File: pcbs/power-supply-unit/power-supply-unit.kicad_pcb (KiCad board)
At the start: 2 copper layers, 34.3 x 83.2 mm, 23 parts, among them J1 BMS_OUTPUT, J2 PWR_CONN_RASPI, J3 PWR_CONN_CTRL, U1 LM2576S-ADJ, U2 LM2576S-ADJ, U3 AMS1117-3.3

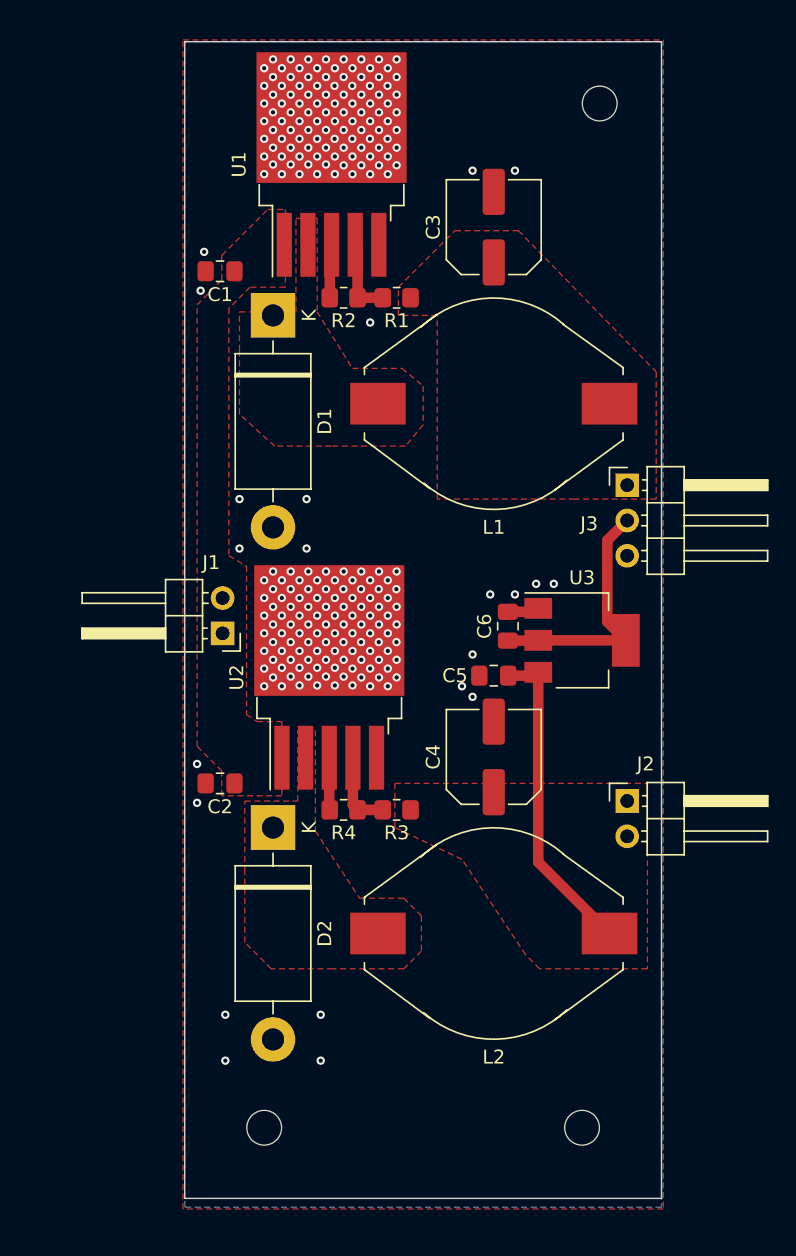
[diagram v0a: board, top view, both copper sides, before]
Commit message: Redesign PWR supply to match real part footprints
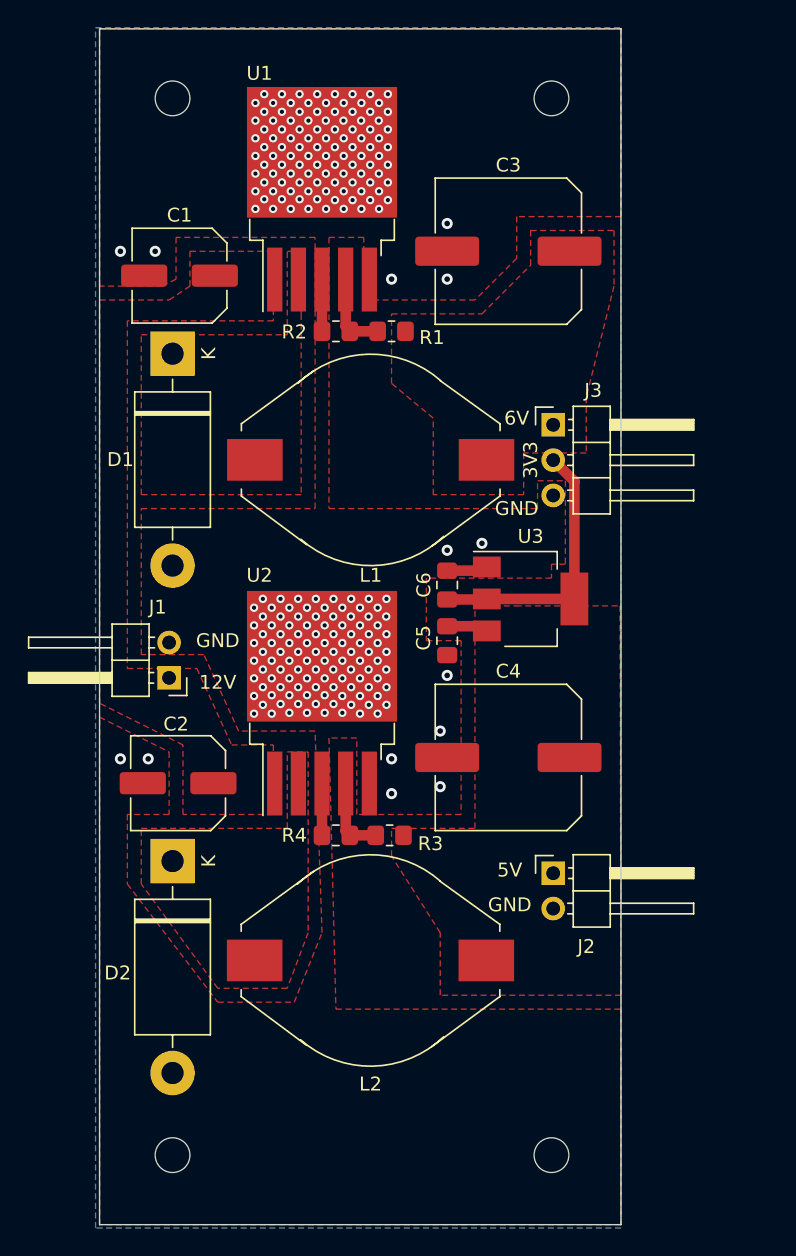
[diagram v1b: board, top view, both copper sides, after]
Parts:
- added REF03: MountingHole_2.5mm, MountingHole:MountingHole_2.5mm, F.Cu at (110.2, 39.0)
- C1, C2: footprint Capacitor_SMD:C_0805_2012Metric_Pad1.18x1.45mm_HandSolder -> Capacitor_SMD:C_Elec_6.3x7.7
- C3, C4: footprint Capacitor_SMD:C_Elec_6.3x7.7 -> Capacitor_SMD:C_Elec_10x10.2
- moved L1 9.73 mm to (124.5, 65.0)
- moved L2 9.07 mm to (124.5, 101.0)
- moved D1 7.73 mm to (110.2, 57.4)
- moved D2 7.62 mm to (110.2, 93.9)
- moved J2 7.44 mm to (137.6, 94.7)
- moved REF02 6.88 mm to (110.2, 115.0)
- moved J3 6.87 mm to (137.6, 62.5)
- moved C6 5.28 mm to (130.0, 74.0)
- moved J1 5.01 mm to (110.0, 80.7)
- moved U3 4.75 mm to (136.0, 75.0)
- moved C5 4.19 mm to (130.0, 78.0), turned to -90 degrees
- moved REF03 3.49 mm to (137.5, 39.0)
- moved C2 3.02 mm to (110.6, 88.2)
- moved REF01 2.95 mm to (137.5, 115.0)
- moved C1 2.93 mm to (110.8, 51.8)
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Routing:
- net +5V: track 23.2 -> 2.99 mm
- net +3V3: track 18.3 -> 19.8 mm
- net GND: track 9.91 -> 10.4 mm, vias 246 -> 238
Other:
- board size 34.3 x 83.2 mm -> 37.5 x 86 mm
- board text added: "12V"
- board text added: "3V3"
- board text added: "5V"
- board text added: "6V"
- board text added: "GND"

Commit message: Fix small errors, add more stitching vias
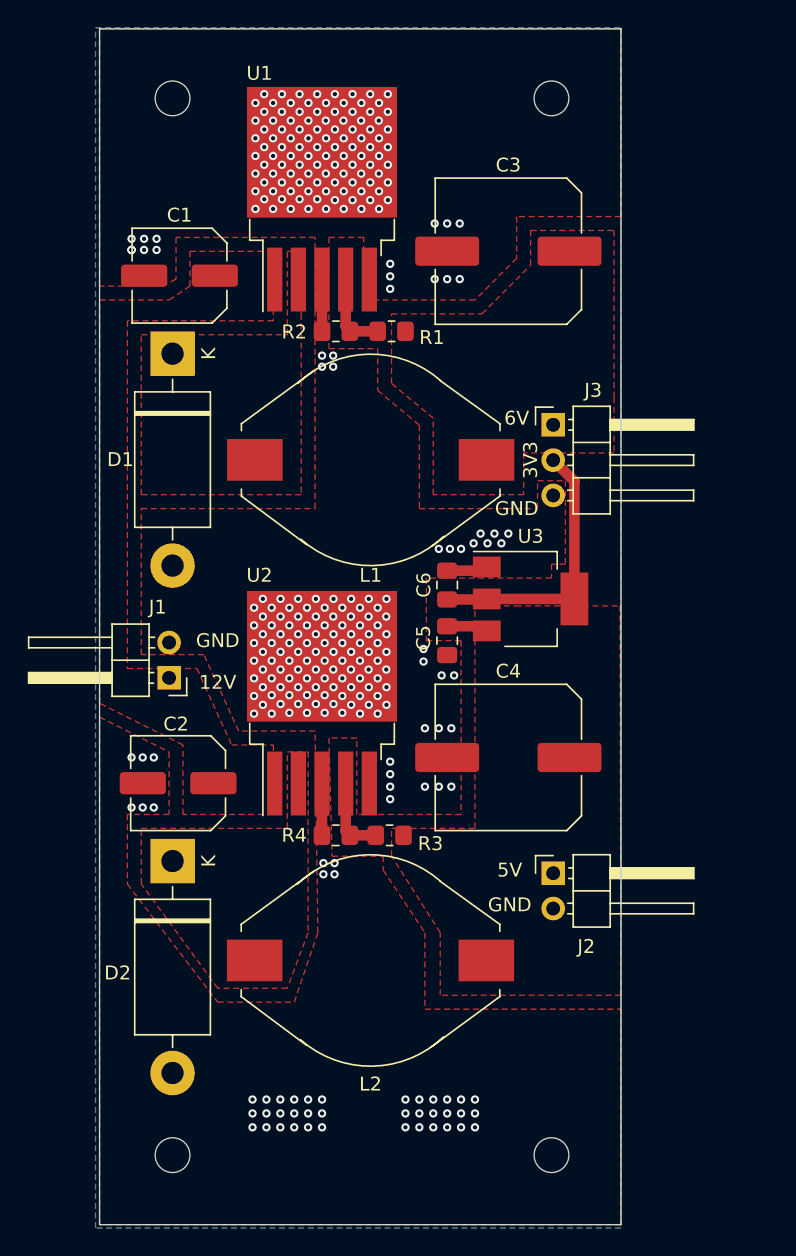
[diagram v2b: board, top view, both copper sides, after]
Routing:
- net GND: vias 238 -> 313
